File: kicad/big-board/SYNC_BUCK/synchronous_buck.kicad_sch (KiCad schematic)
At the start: 33 parts, among them J9 Conn_01x04, Q1 PSMQC092N10LS1, Q2 PSMQC076N12LS1, U4 UCC27282DRCR, U5 NCS214RMUTAG

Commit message: Update PCB
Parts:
- C16: footprint Capacitor_SMD:C_0805_2012Metric_Pad1.18x1.45mm_HandSolder -> Capacitor_SMD:C_1206_3216Metric
- R16: footprint Resistor_SMD:R_0805_2012Metric -> Resistor_SMD:R_1206_3216Metric_Pad1.30x1.75mm_HandSolder
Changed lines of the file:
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@@
       (effects (font (size 1.27 1.27)) (justify left))
     )
-    (property "Footprint" "Resistor_SMD:R_0805_2012Metric" (id 2) (at 156.972 127 90)
+    (property "Footprint" "Resistor_SMD:R_1206_3216Metric_Pad1.30x1.75mm_HandSolder" (id 2) (at 156.972 127 90)
       (effects (font (size 1.27 1.27)) hide)
     )
@@
       (effects (font (size 1.27 1.27)) (justify left))
     )
-    (property "Footprint" "Capacitor_SMD:C_0805_2012Metric_Pad1.18x1.45mm_HandSolder" (id 2) (at 159.7152 143.51 0)
+    (property "Footprint" "Capacitor_SMD:C_1206_3216Metric" (id 2) (at 159.7152 143.51 0)
       (effects (font (size 1.27 1.27)) hide)
     )

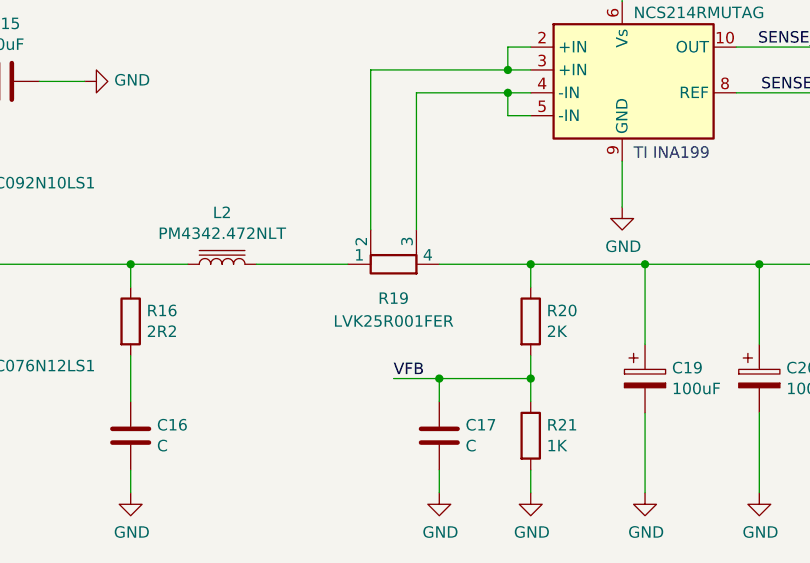
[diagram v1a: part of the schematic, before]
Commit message: Update PCB
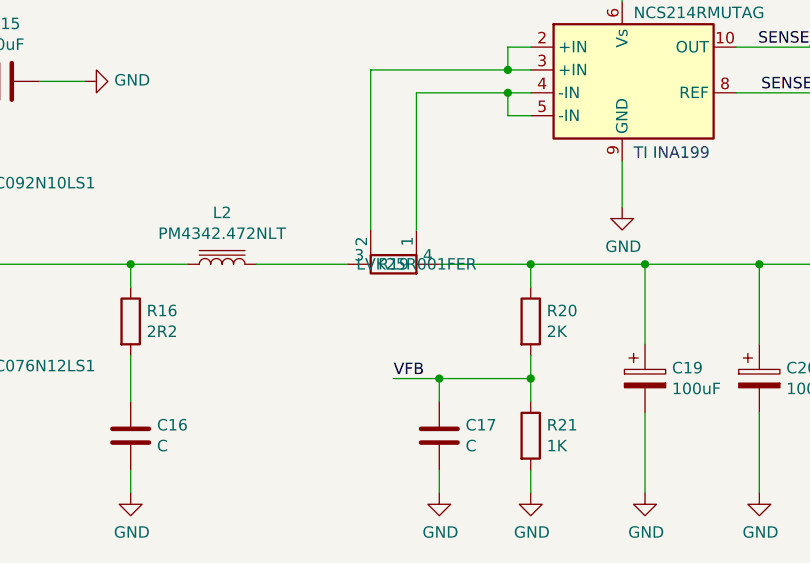
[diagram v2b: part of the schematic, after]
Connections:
- net at L2.2: now also R19.3; no longer R19.1
- net at U5.4 (-IN), U5.5 (-IN): now also R19.1; no longer R19.3
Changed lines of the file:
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@@
   )
   (symbol (lib_id "Device:R_Shunt") (at 187.96 120.65 90) (unit 1)
-    (in_bom yes) (on_board yes) (fields_autoplaced)
-    (property "Reference" "R19" (id 0) (at 187.96 124.46 90))
-    (property "Value" "LVK25R001FER" (id 1) (at 187.96 127 90))
-    (property "Footprint" "Resistor_SMD:R_Shunt_Ohmite_LVK25" (id 2) (at 187.96 122.428 90)
+    (in_bom yes) (on_board yes)
+    (property "Reference" "R19" (id 0) (at 187.96 120.65 90))
+    (property "Value" "LVK25R001FER" (id 1) (at 190.5 120.65 90))
+    (property "Footprint" "Resistor_SMD:R_Shunt_Ohmite_LVK25" (id 2) (at 186.182 120.65 90)
       (effects (font (size 1.27 1.27)) hide)
     )
@@
       (effects (font (size 1.27 1.27)) hide)
     )
+    (pin "2")
     (pin "1")
-    (pin "2")
     (pin "3")
     (pin "4")
